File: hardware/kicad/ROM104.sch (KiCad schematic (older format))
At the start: 43 parts, among them J1 Screw_Terminal_01x12, J2 CAN, K1 DIPxx-1Cxx-51x, K2 DIPxx-1Cxx-51x, K3 DIPxx-1Cxx-51x, K4 DIPxx-1Cxx-51x, SW1 INSTANCE, SW2 BUS, U1 L293D, U2 MCP2551-I-P, U3 TMR-1211, U4 Teensy_3.2, U5 L293D

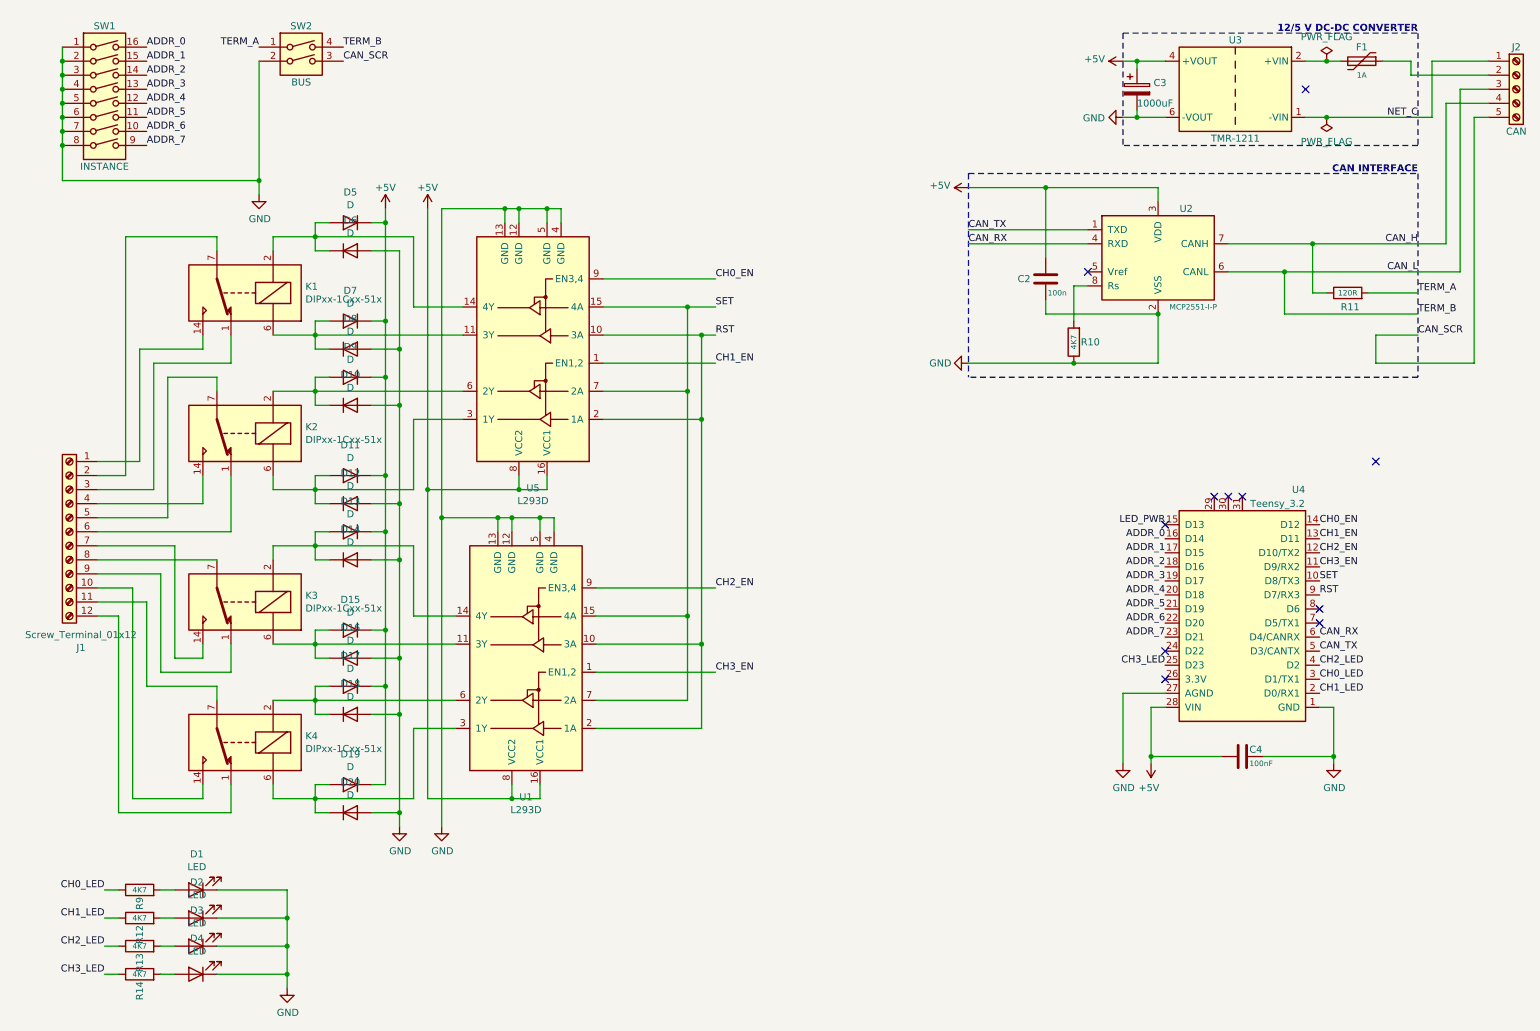
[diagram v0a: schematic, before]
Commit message: Stuff
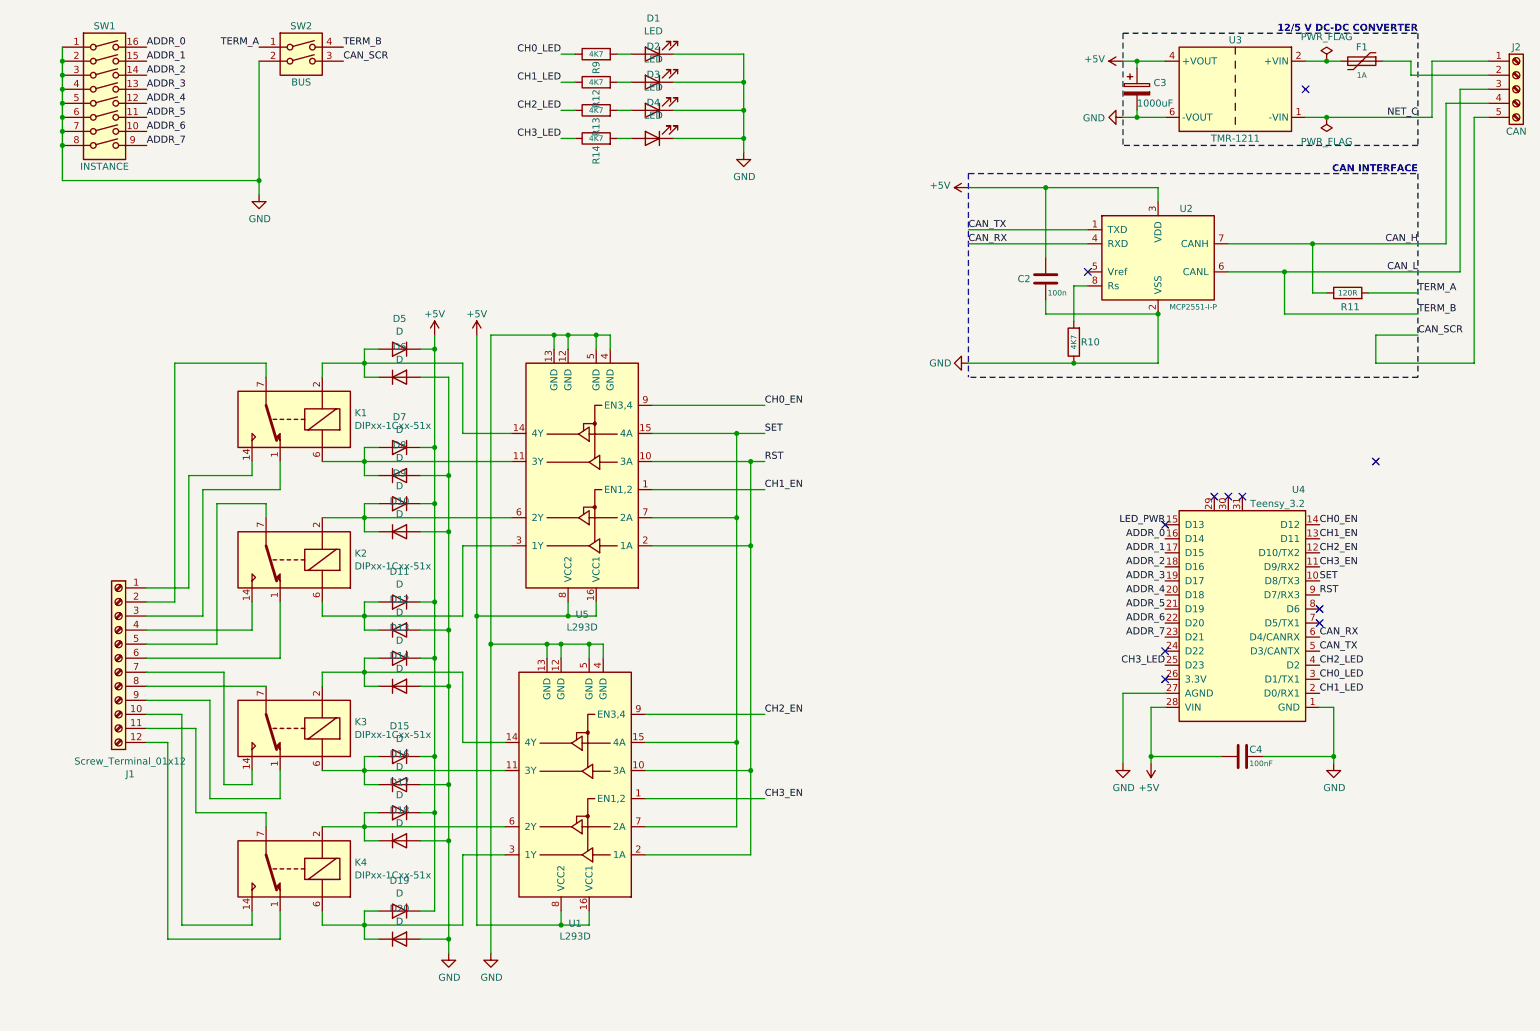
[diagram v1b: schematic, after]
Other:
- moved on the sheet: D1, D10, D11, D12, D13, D14, D15, D16, D17, D18, D19, D2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

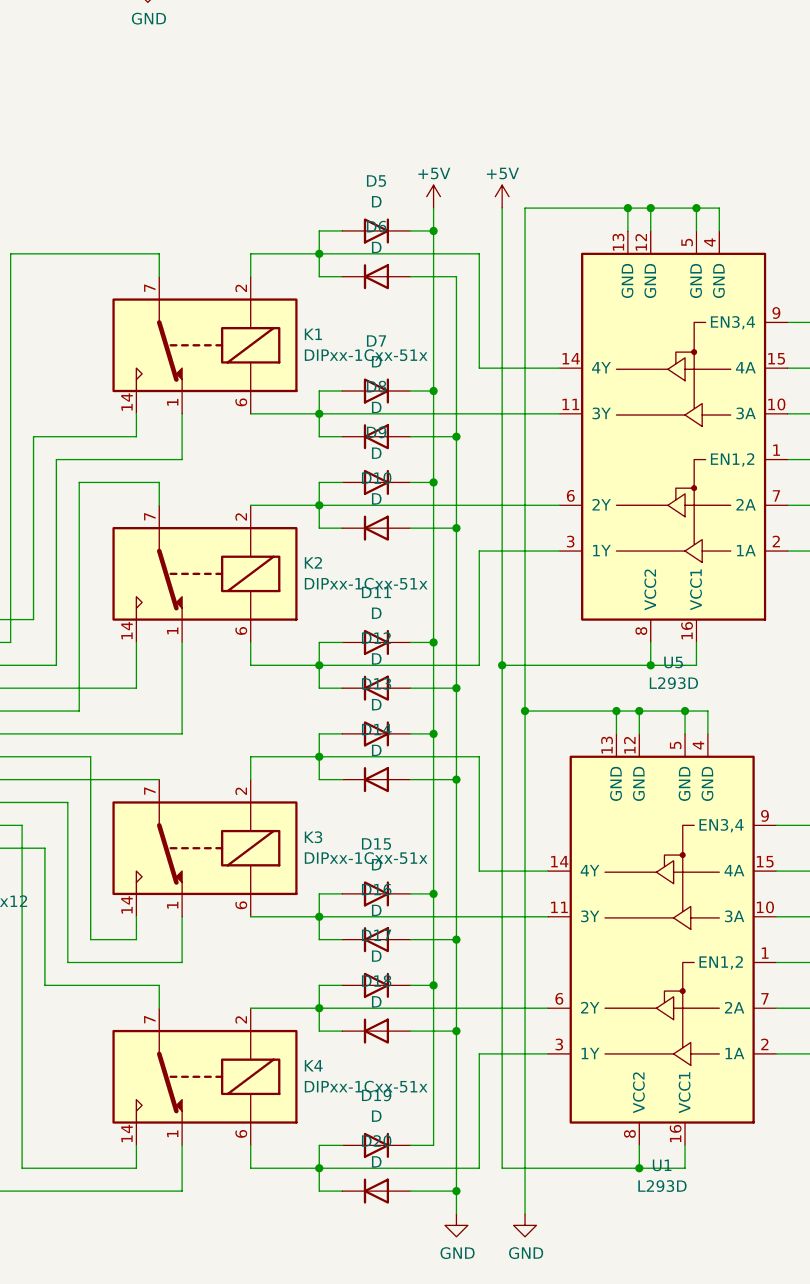
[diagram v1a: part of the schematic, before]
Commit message: Tweaks
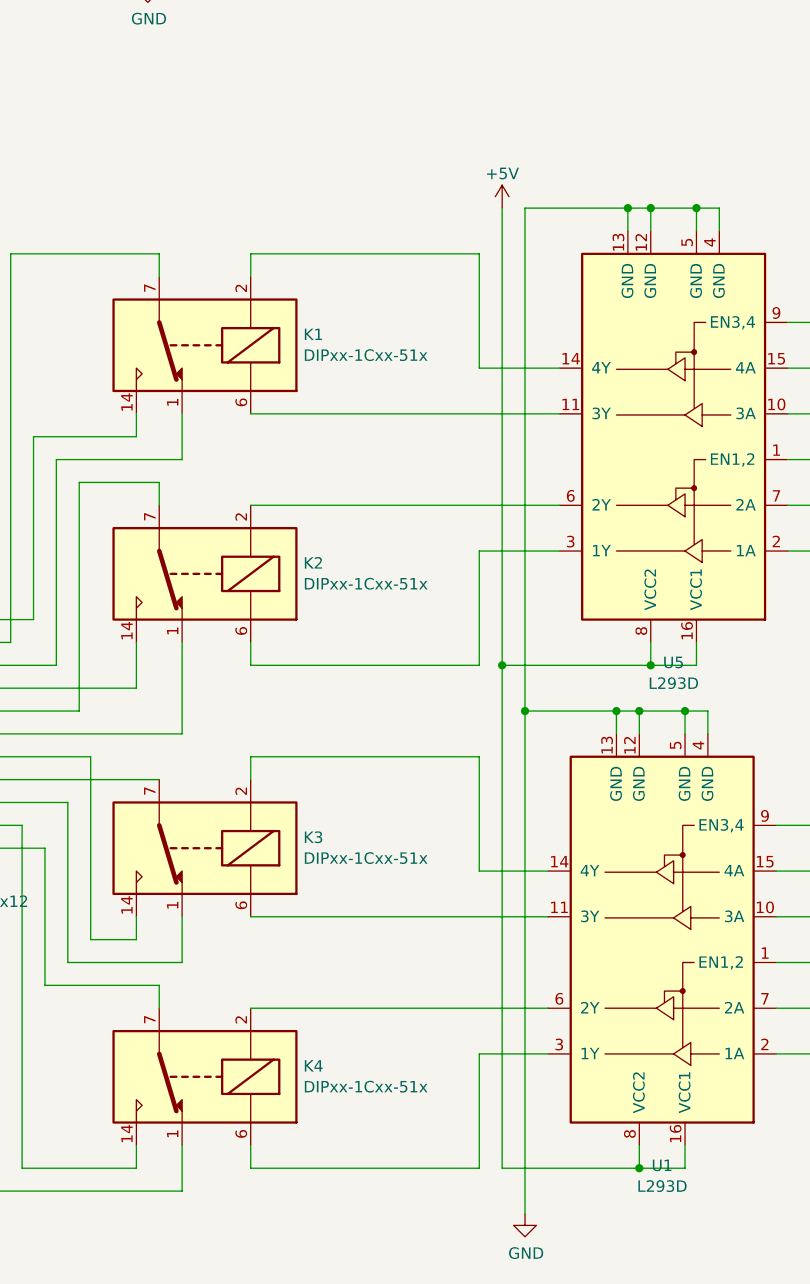
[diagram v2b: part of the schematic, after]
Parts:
- removed D10, D11, D12, D13, D14, D15, D16, D17, D18, D19, D20, D5, D6, D7, D8, D9: D, Diode_THT:D_A-405_P2.54mm_Vertical_AnodeUp, symbol Device:D

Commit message: Stuff
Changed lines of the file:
@@
 	3450 5200 3450 5700
 Wire Wire Line
-	4200 4800 4200 4700
-Wire Wire Line
-	4400 4800 4400 4700
-Wire Wire Line
-	4150 6900 4150 7000
-Wire Wire Line
 	4150 7000 4350 7000
-Wire Wire Line
-	4350 7000 4350 6900
 Wire Wire Line
 	3550 4800 3550 7000
@@
 Wire Wire Line
 	4100 2800 3650 2800
-Wire Wire Line
-	3650 2800 3650 5000
 Connection ~ 4100 2800
 $Comp
@@
 Connection ~ 4050 5000
 Connection ~ 3650 5000
-Wire Wire Line
-	3650 5000 3650 7200
 Text Label 5600 6100 0    50   ~ 0
 CH3_EN
@@
 Wire Wire Line
 	2450 7000 3450 7000
+Wire Wire Line
+	4200 4700 4200 4800
+Wire Wire Line
+	4400 4700 4400 4800
+Wire Wire Line
+	3650 2800 3650 5000
+Wire Wire Line
+	4350 6900 4350 7000
+Wire Wire Line
+	4150 6900 4150 7000
+Wire Wire Line
+	3650 5000 3650 7200
 $EndSCHEMATC

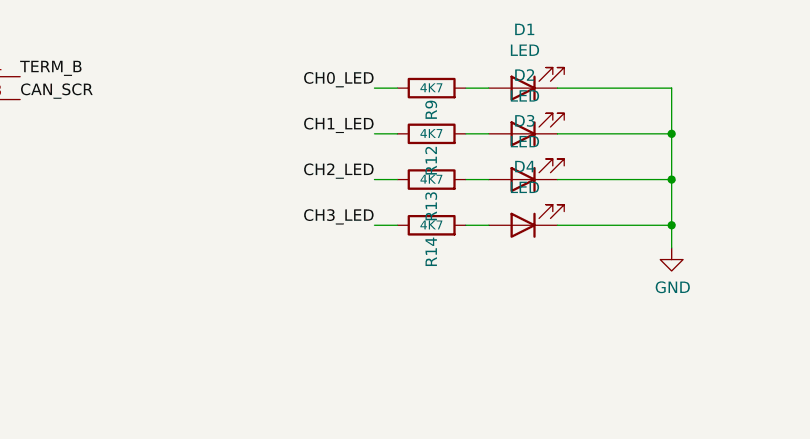
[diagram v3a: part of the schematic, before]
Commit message: Tweaks
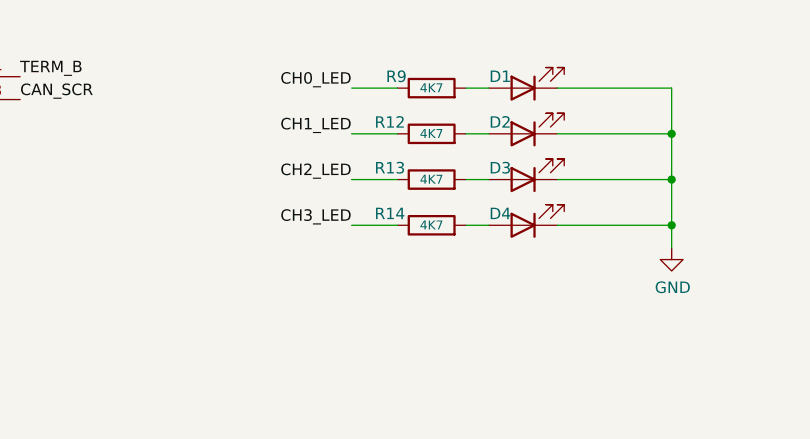
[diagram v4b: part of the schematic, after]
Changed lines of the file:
@@
 U 1 1 631C1A0C
 P 4400 800
-F 0 "R9" H 4350 800 50  0000 R CNN
+F 0 "R9" V 4450 1000 50  0000 R CNN
 F 1 "4K7" V 4400 800 39  0000 C CNN
 F 2 "Resistor_THT:R_Axial_DIN0204_L3.6mm_D1.6mm_P5.08mm_Horizontal" V 4330 800 50  0001 C CNN
@@
 U 1 1 631C329D
 P 4800 800
-F 0 "D1" H 4793 545 50  0000 C CNN
-F 1 "LED" H 4793 636 50  0000 C CNN
+F 0 "D1" H 4900 750 50  0000 C CNN
+F 1 "LED" H 4793 636 50  0001 C CNN
 F 2 "LED_THT:LED_D1.8mm_W3.3mm_H2.4mm" H 4800 800 50  0001 C CNN
 F 3 "~" H 4800 800 50  0001 C CNN
@@
 	4550 800  4650 800
 Wire Wire Line
-	4150 800  4250 800
+	4050 800  4250 800
 Wire Wire Line
 	4950 800  5450 800
@@
 U 1 1 631D6F98
 P 4400 1000
-F 0 "R12" H 4350 1000 50  0000 R CNN
+F 0 "R12" V 4450 1250 50  0000 R CNN
 F 1 "4K7" V 4400 1000 39  0000 C CNN
 F 2 "Resistor_THT:R_Axial_DIN0204_L3.6mm_D1.6mm_P5.08mm_Horizontal" V 4330 1000 50  0001 C CNN
@@
 U 1 1 631D739B
 P 4400 1200
-F 0 "R13" H 4350 1200 50  0000 R CNN
+F 0 "R13" V 4450 1450 50  0000 R CNN
 F 1 "4K7" V 4400 1200 39  0000 C CNN
 F 2 "Resistor_THT:R_Axial_DIN0204_L3.6mm_D1.6mm_P5.08mm_Horizontal" V 4330 1200 50  0001 C CNN
@@
 U 1 1 631D7696
 P 4400 1400
-F 0 "R14" H 4350 1400 50  0000 R CNN
+F 0 "R14" V 4450 1650 50  0000 R CNN
 F 1 "4K7" V 4400 1400 39  0000 C CNN
 F 2 "Resistor_THT:R_Axial_DIN0204_L3.6mm_D1.6mm_P5.08mm_Horizontal" V 4330 1400 50  0001 C CNN
@@
 U 1 1 631D7AEF
 P 4800 1000
-F 0 "D2" H 4793 745 50  0000 C CNN
-F 1 "LED" H 4793 836 50  0000 C CNN
+F 0 "D2" H 4900 950 50  0000 C CNN
+F 1 "LED" H 4793 836 50  0001 C CNN
 F 2 "LED_THT:LED_D1.8mm_W3.3mm_H2.4mm" H 4800 1000 50  0001 C CNN
 F 3 "~" H 4800 1000 50  0001 C CNN
@@
 U 1 1 631D7EE7
 P 4800 1200
-F 0 "D3" H 4793 945 50  0000 C CNN
-F 1 "LED" H 4793 1036 50  0000 C CNN
+F 0 "D3" H 4900 1150 50  0000 C CNN
+F 1 "LED" H 4793 1036 50  0001 C CNN
 F 2 "LED_THT:LED_D1.8mm_W3.3mm_H2.4mm" H 4800 1200 50  0001 C CNN
 F 3 "~" H 4800 1200 50  0001 C CNN
@@
 U 1 1 631D8355
 P 4800 1400
-F 0 "D4" H 4793 1145 50  0000 C CNN
-F 1 "LED" H 4793 1236 50  0000 C CNN
+F 0 "D4" H 4900 1350 50  0000 C CNN
+F 1 "LED" H 4793 1236 50  0001 C CNN
 F 2 "LED_THT:LED_D1.8mm_W3.3mm_H2.4mm" H 4800 1400 50  0001 C CNN
 F 3 "~" H 4800 1400 50  0001 C CNN
@@
 $EndComp
 Wire Wire Line
-	4150 1000 4250 1000
+	4050 1000 4250 1000
 Wire Wire Line
-	4150 1200 4250 1200
+	4050 1200 4250 1200
 Wire Wire Line
-	4150 1400 4250 1400
-Text Label 4150 800  2    50   ~ 0
+	4050 1400 4250 1400
+Text Label 4050 800  2    50   ~ 0
 CH0_LED
-Text Label 4150 1000 2    50   ~ 0
+Text Label 4050 1000 2    50   ~ 0
 CH1_LED
-Text Label 4150 1200 2    50   ~ 0
+Text Label 4050 1200 2    50   ~ 0
 CH2_LED
-Text Label 4150 1400 2    50   ~ 0
+Text Label 4050 1400 2    50   ~ 0
 CH3_LED
 $Comp
